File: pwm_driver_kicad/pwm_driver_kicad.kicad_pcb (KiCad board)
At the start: 2 copper layers, 35 x 35 mm, 10 parts, among them J1 Bornera, Q1 IRF1407, U1 NE555P

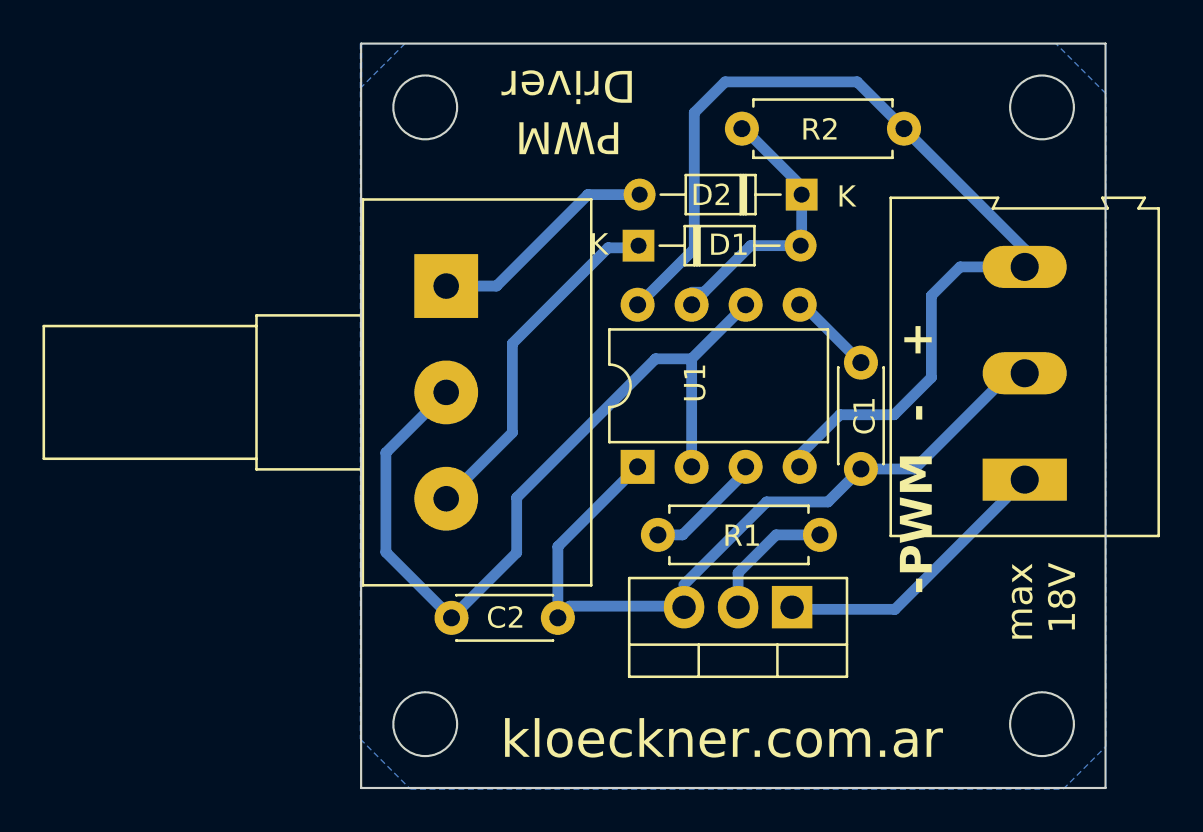
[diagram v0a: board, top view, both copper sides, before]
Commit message: update schematic resistor values | fix simulation
NOTE: the pcb has **not** been updated yet
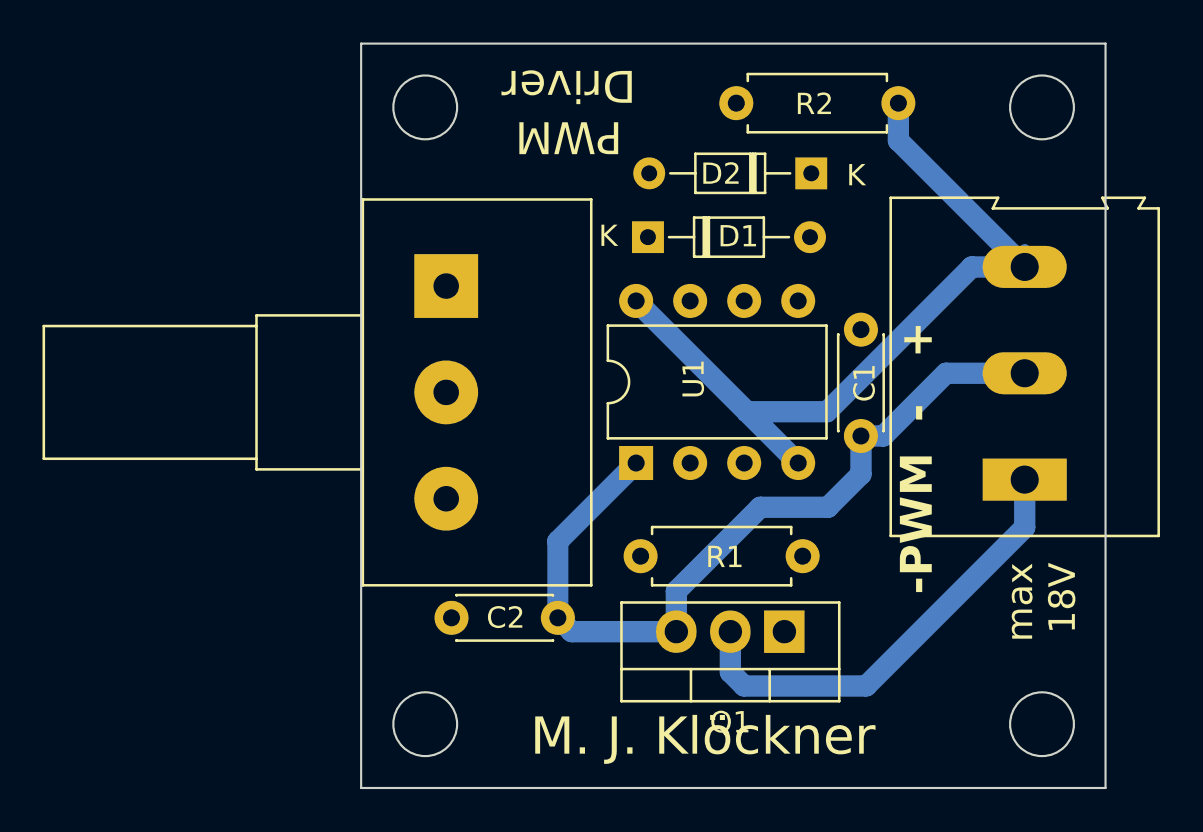
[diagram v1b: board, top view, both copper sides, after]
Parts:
- Q1: footprint Package_TO_SOT_THT:TO-220-3_Vertical -> Library:TO-220-3_Vertical_G_D_S_order
- moved C1 1.55 mm to (128.5, 58.5)
- moved R1 1.29 mm to (118.1, 69.1)
- moved R2 1.23 mm to (130.2, 47.8)
- moved Q1 1.21 mm to (124.9, 72.7)
- moved D2 1.10 mm to (126.2, 51.1)
- moved D1 0.60 mm to (118.5, 54.1)
- moved U1 0.19 mm to (117.9, 64.7)
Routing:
- net Net-(U1-THR): track 39.6 -> 0.00 mm
- net Net-(D1-K): track 16.8 -> 0.00 mm
- net Net-(D1-A): track 13.0 -> 0.55 mm
- net Net-(D2-A): track 11.3 -> 0.00 mm
- net VCC: track 47.8 -> 38.6 mm
- net Net-(J1-Pin_3): track 14.0 -> 21.3 mm
- net Net-(Q1-G): track 6.00 -> 0.00 mm
- net Net-(U1-Q): track 5.71 -> 0.12 mm
- net Net-(U1-CV): track 4.01 -> 0.16 mm
- net 0: track 35.3 -> 38.9 mm
- removed copper zone on B.Cu, net 0
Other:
- board text added: "M. J. Klöckner"
- board text removed: "kloeckner.com.ar"
